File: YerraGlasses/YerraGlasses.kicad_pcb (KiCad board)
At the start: 4 copper layers, 68 x 21.5 mm, 28 parts, among them J1 Conn_01x02_Pin, J11 USB_C_Receptacle_USB2.0_16P, J2 Conn_01x02_Pin, J3 Conn_01x02_Pin, J4 Conn_01x02_Pin, J5 Conn_01x02_Pin, SW1 SW_SPDT, U1 ESP32-S3-WROOM-1, U2 MAX98357A, U3 MAX98357A, U4 RT9013-33GB

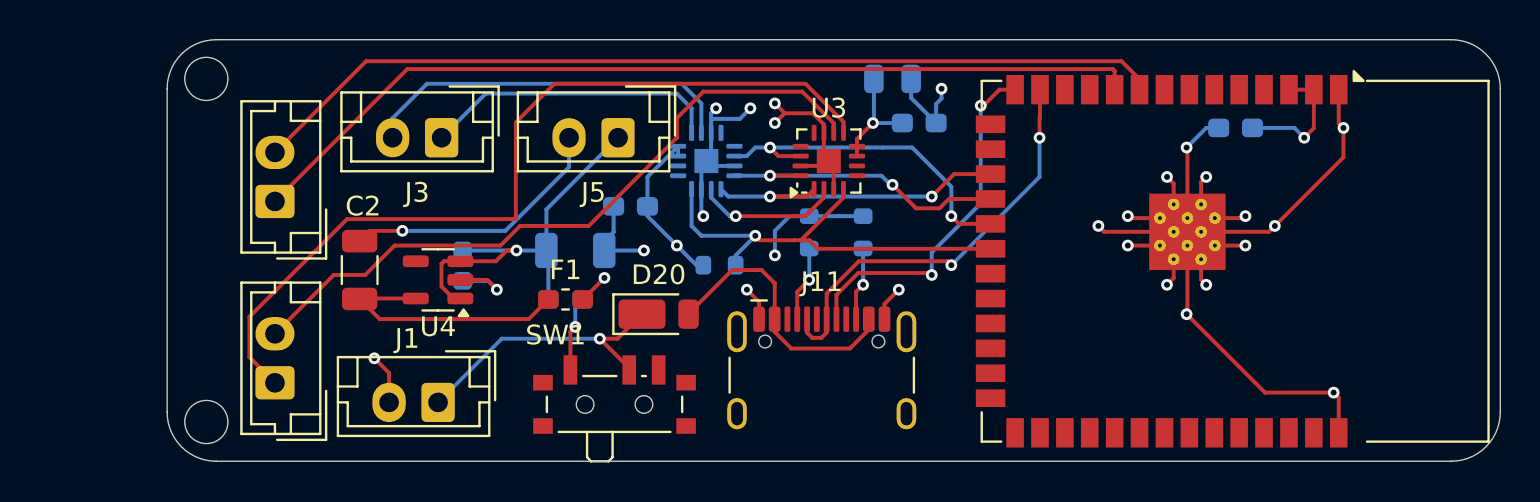
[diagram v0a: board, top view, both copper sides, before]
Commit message: cad completion prototype
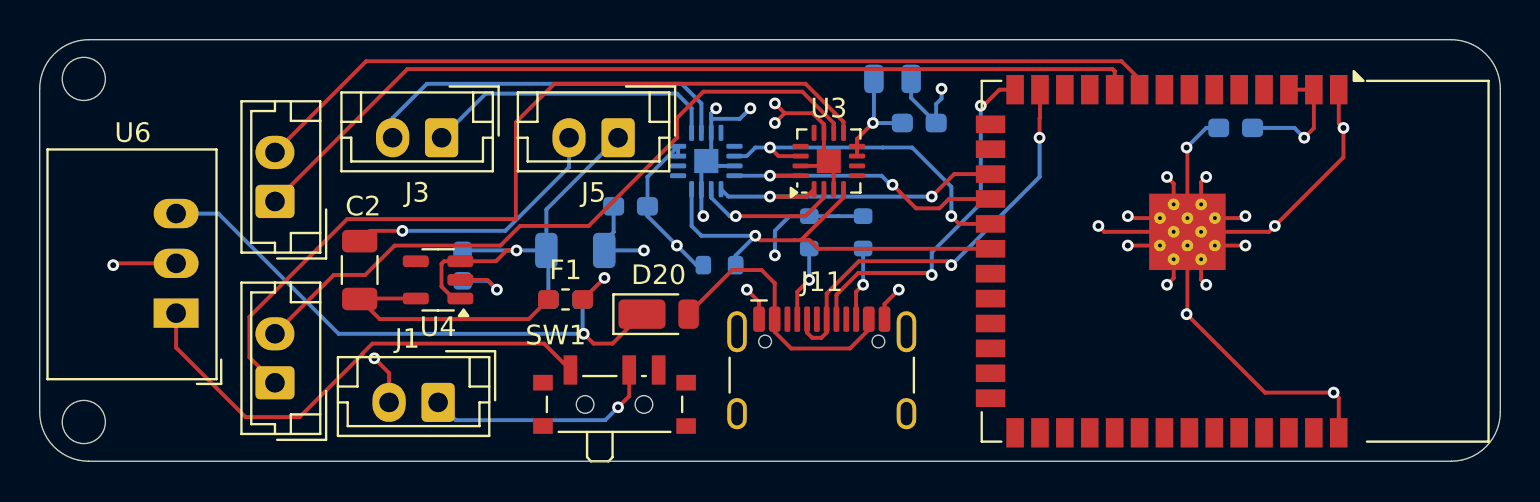
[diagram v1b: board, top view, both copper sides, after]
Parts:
- removed the REF** at (166.0, 43.0)
- removed the REF** at (166.0, 60.5)
- added ?: , , F.Cu at (159.8, 60.5)
- added REF**: MountingHole_2.2mm_M2_custom, MountingHole:MountingHole_2.2mm_M2_custom, F.Cu at (159.8, 43.0)
- added U6: R-78E5.0-1.0, Converter_DCDC:Converter_DCDC_RECOM_R-78E-0.5_THT, F.Cu at (164.5, 54.9)
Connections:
- D20 pad 1: /Connectors/5V_unfused -> /Power/5V_unfused
- F2 pad 1: Net-(SW1-A) -> /Power/5V_unfused
- J1 pad 1: /Connectors/5V_unfused -> /Connectors/9V_unfused
- SW1 pad 2: /Connectors/5V_unfused -> /Connectors/9V_unfused
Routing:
- net /Power/5V_unfused: track 0.00 -> 29.4 mm, vias 0 -> 1
- net Net-(SW1-A): track 3.85 -> 25.5 mm, vias 1 -> 0
- net /Connectors/5V_unfused: track 14.5 -> 0.00 mm, vias 1 -> 0
- net /Connectors/9V_unfused: track 0.00 -> 12.1 mm, vias 0 -> 1
- net GND: track 107.4 -> 110.6 mm, vias 27 -> 28
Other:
- board size 68 x 21.5 mm -> 74.5 x 21.5 mm
